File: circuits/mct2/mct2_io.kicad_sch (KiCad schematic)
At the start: 125 parts

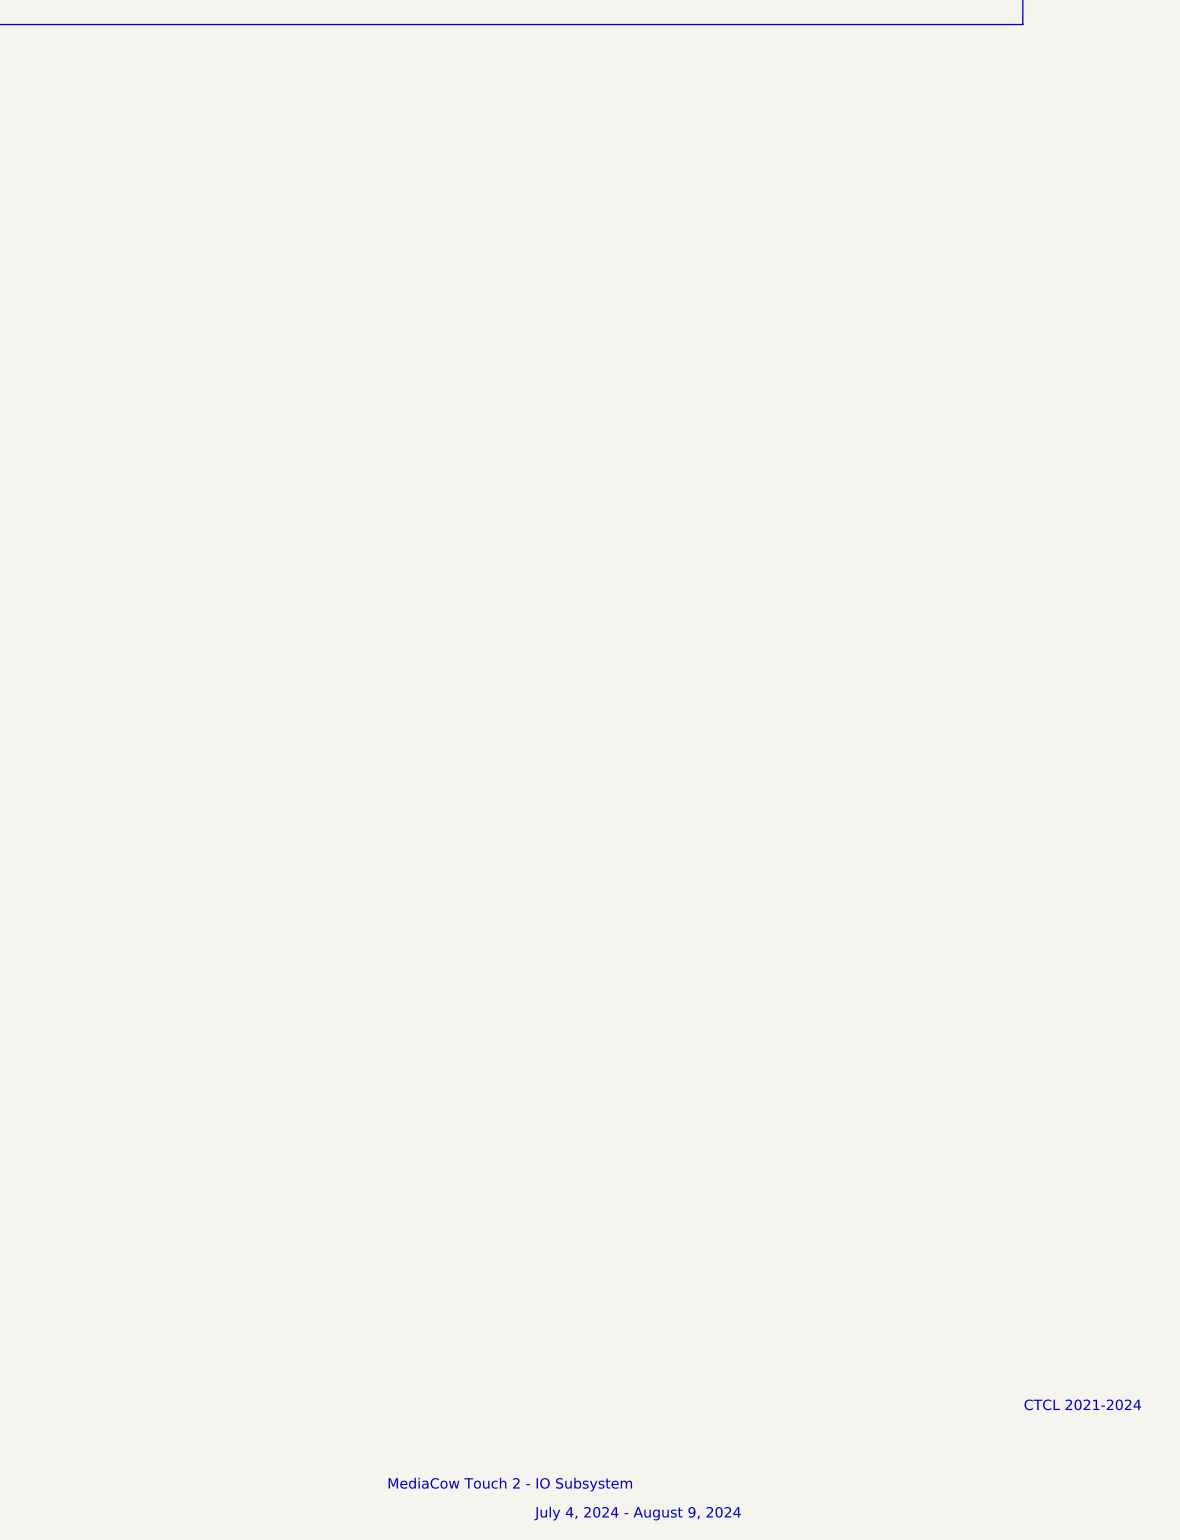
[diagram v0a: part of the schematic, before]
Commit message: Aug 11, 2024 2
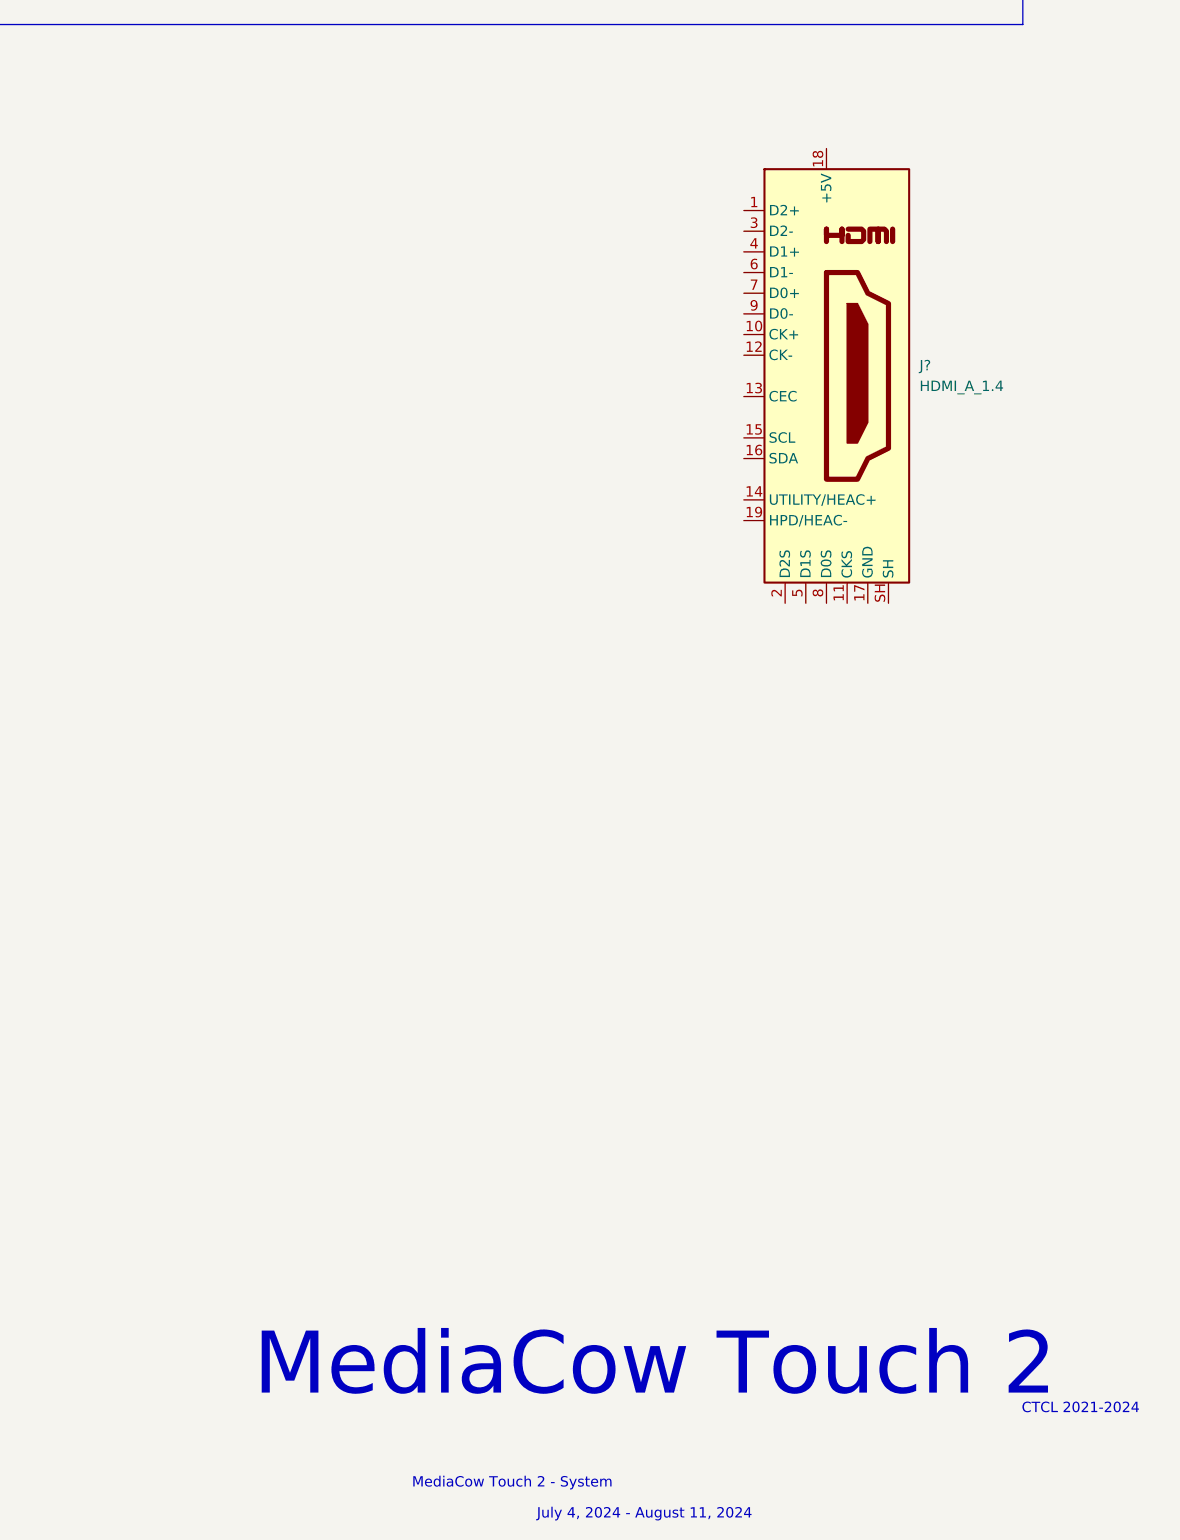
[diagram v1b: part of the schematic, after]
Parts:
- added J?: HDMI_A_1.4, symbol Connector:HDMI_A_1.4
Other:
- note added: "July 4, 2024 - August 11, 2024"
- note added: "MediaCow Touch 2"
- note added: "MediaCow Touch 2 - System"
- note removed: "July 4, 2024 - August 9, 2024"
- note removed: "MediaCow Touch 2 - IO Subsystem"
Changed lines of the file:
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@@
 		)
 	)
-	(text "July 4, 2024 - August 9, 2024"
+	(text "MediaCow Touch 2 - System"
 		(exclude_from_sim no)
-		(at 1113.536 824.484 0)
+		(at 1098.042 820.674 0)
 		(effects
 			(font
@@
 		)
 	)
-	(text "MediaCow Touch 2 - IO Subsystem\n"
+	(text "MediaCow Touch 2"
 		(exclude_from_sim no)
-		(at 1097.788 820.928 0)
+		(at 1115.568 806.196 0)
+		(effects
+			(font
+				(face "Heuristica")
+				(size 7.62 7.62)
+			)
+		)
+	)
+	(text "July 4, 2024 - August 11, 2024"
+		(exclude_from_sim no)
+		(at 1114.298 824.484 0)
 		(effects
 			(font
@@
 	(text "CTCL 2021-2024"
 		(exclude_from_sim no)
-		(at 1168.146 811.276 0)
+		(at 1167.892 811.53 0)
 		(effects
 			(font
@@
 					(unit 1)
 				)
+			)
+		)
+	)
+	(symbol
+		(lib_id "Connector:HDMI_A_1.4")
+		(at 1136.65 684.53 0)
+		(unit 1)
+		(exclude_from_sim no)
+		(in_bom yes)
+		(on_board yes)
+		(dnp no)
+		(fields_autoplaced yes)
+		(property "Reference" "J?"
+			(at 1148.08 683.2599 0)
+			(effects
+				(font
+					(size 1.27 1.27)
+				)
+				(justify left)
+			)
+		)
+		(property "Value" "HDMI_A_1.4"
+			(at 1148.08 685.7999 0)
+			(effects
+				(font
+					(size 1.27 1.27)
+				)
+				(justify left)
+			)
+		)
+		(property "Footprint" ""
+			(at 1137.285 684.53 0)
+			(effects
+				(font
+					(size 1.27 1.27)
+				)
+				(hide yes)
+			)
+		)
+		(property "Datasheet" "https://en.wikipedia.org/wiki/HDMI"
+			(at 1137.285 684.53 0)
+			(effects
+				(font
+					(size 1.27 1.27)
+				)
+				(hide yes)
+			)
+		)
+		(property "Description" "HDMI 1.4+ type A connector"
+			(at 1136.65 684.53 0)
+			(effects
+				(font
+					(size 1.27 1.27)
+				)
+				(hide yes)
+			)
+		)
+		(pin "14"
+		)
+		(pin "2"
+		)
+		(pin "9"
+		)
+		(pin "13"
+		)
+		(pin "SH"
+		)
+		(pin "1"
+		)
+		(pin "8"
+		)
+		(pin "18"
+		)
+		(pin "19"
+		)
+		(pin "12"
+		)
+		(pin "7"
+		)
+		(pin "10"
+		)
+		(pin "6"
+		)
+		(pin "11"
+		)
+		(pin "5"
+		)
+		(pin "15"
+		)
+		(pin "16"
+		)
+		(pin "17"
+		)
+		(pin "4"
+		)
+		(pin "3"
+		)
+		(instances
+			(project ""
+				(path "/0917e100-0497-47cd-9e32-3e43ad224d2b/c9720429-3bf3-4c3a-9e7d-2ba35698ba31"
+					(reference "J?")
+					(unit 1)
+				)

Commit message: Aug 13, 2024
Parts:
- removed C? (x4): 100nF, symbol Device:C_Small
- removed J?: USB_A_Stacked, symbol Connector:USB_A_Stacked
- removed R? (x2): 20K, symbol Device:R_Small
- removed R? (x2): 56K, symbol Device:R_Small
- removed U? (x2): TPS25221, symbol mediacow:TPS25221
- removed U? (x2): TPD4EUSB30, Package_TO_SOT_SMD:Texas_DRT-3, symbol mediacow:TPD2EUSB30
- added C? (x10): 220nF, symbol Device:C_Small
- added C? (x14): 100nF, symbol Device:C_Small
- added C? (x4): 10uF, symbol Device:C_Small
- added J?: Bus_M.2_Socket_E, symbol Connector:Bus_M.2_Socket_E
- added J?: Bus_M.2_Socket_M, symbol Connector:Bus_M.2_Socket_M
- added R? (x4): 0, symbol Device:R_Small
- added R? (x2): 10K, symbol Device:R_Small
- added U?: TPD4EUSB30, Package_TO_SOT_SMD:Texas_DRT-3, symbol mediacow:TPD2EUSB30
- added U?: TPD12S016RKTR, RKT24, symbol mediacow:TPD12S016RKTR
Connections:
- net GND: now also J?.11 (CKS), J?.17 (GND), J?.2 (D2S), J?.5 (D1S), J?.8 (D0S), J?.SH, C?.1, C?.1, C?.2, C?.2, C?.2, C?.2, C?.2, C?.2, C?.2, C?.2, J?.1 (GND), J?.1 (GND), J?.15 (GND), J?.18 (GND), J?.21 (GND), J?.27 (GND), J?.3 (GND), J?.33 (GND), J?.33 (GND), J?.39 (GND), J?.39 (GND), J?.45 (GND), J?.45 (GND), J?.51 (GND), J?.51 (GND), J?.57 (GND), J?.57 (GND), J?.63 (GND), J?.69 (GND), J?.7 (GND), J?.71 (GND), J?.73 (GND), J?.75 (GND), J?.75 (GND), J?.9 (GND), R?.1, R?.1, U?.13 (GND), U?.18 (GND), U?.3 (GND), U?.5 (GND)
- net LAN_0V9: now also U?.11 (VDD0p9), U?.32 (VDD0p9), U?.42 (VDD0p9), U?.59 (VDD0p9)
- net LAN_1V5: now also U?.47 (VDD1p5), U?.56 (VDD1p5)
- net at J?.1 (D2+): now also C?.1
- net at J?.10 (CK+): now also C?.1
- net at J?.12 (CK-): now also C?.1
- net DDIB_SCL_CN: now reaches J?.15 (SCL)
- net DDIB_SCL_CN: now also U?.7 (SCL_B)
- net DDIB_SDA_CN: now reaches J?.16 (SDA)
- net DDIB_SDA_CN: now also U?.8 (SDA_B)
- net DDIB_5V_CN: now reaches J?.18 (+5V)
- net DDIB_5V_CN: now also C?.2, U?.12 (5V_OUT)
- net DDIB_HPD_CN: now reaches J?.19 (HPD/HEAC-)
- net DDIB_HPD_CN: now also U?.9 (HPD_B)
- net at J?.3 (D2-): now also C?.1
- net at J?.4 (D1+): now also C?.1
- net at J?.6 (D1-): now also C?.1
- net at J?.7 (D0+): now also C?.1
- net at J?.9 (D0-): now also C?.1
- new net: J?.53 (~{CLKREQ0}), R?.2
- new net: C?.2, J?.37 (PETp1)
- new net: C?.2, J?.35 (PETn1)
- new net: C?.2, J?.13 (PETp3)
- new net: C?.2, J?.37 (PETn0)
- new net: J?.54 (~{W_DISABLE2}), R?.1
- new net: C?.2, J?.49 (PETp0/SATA-A+)
- new net: C?.2, J?.11 (PETn3)
- new net: J?.56 (~{W_DISABLE1}), R?.1
- new net: J?.68 (SUSCLK), R?.1
- new net: J?.50 (SUSCLK), R?.1
- new net: C?.2, J?.25 (PETp2)
- new net: J?.52 (~{CLKREQ}), R?.2
- new net: C?.2, J?.47 (PETn0/SATA-A-)
- new net: C?.2, J?.35 (PETp0)
- new net: C?.2, J?.23 (PETn2)
- new net DDIB_5V: C?.2, U?.10 (VCC5V)
- new net DDIB_HPD: U?.3 (HPD_A)
- new net DDIB_SCL: U?.1 (SCL_A)
- new net DDIB_SDA: U?.2 (SDA_A)
- new net DDIB_TX0_N: C?.2, U?.21 (D2-)
- new net DDIB_TX0_P: C?.2, U?.22 (D2+)
- new net DDIB_TX1_N: C?.2, U?.19 (D1-)
- new net DDIB_TX1_P: C?.2, U?.20 (D1+)
- new net DDIB_TX2_N: C?.2, U?.16 (D0-)
- new net DDIB_TX2_P: C?.2, U?.17 (D0+)
- new net DDIB_TX3_N: C?.2, U?.14 (CLK-)
- new net DDIB_TX3_P: C?.2, U?.15 (CLK+)
- new net PCIE_M2E_REF_N: J?.49 (REFCLKn0)
- new net PCIE_M2E_REF_P: J?.47 (REFCLKp0)
- new net PCIE_M2E_RX0_N: J?.43 (PERn0)
- new net PCIE_M2E_RX0_P: J?.41 (PERp0)
- new net PCIE_M2E_TX0_N: C?.1
- new net PCIE_M2E_TX0_P: C?.1
- new net PCIE_NVME_REF_N: J?.53 (REFCLKn)
- new net PCIE_NVME_REF_P: J?.55 (REFCLKp)
- new net PCIE_NVME_RX0_N: J?.41 (PERn0/SATA-B+)
- new net PCIE_NVME_RX0_P: J?.43 (PERp0/SATA-B-)
- new net PCIE_NVME_RX1_N: J?.29 (PERn1)
- new net PCIE_NVME_RX1_P: J?.31 (PERp1)
- new net PCIE_NVME_RX2_N: J?.17 (PERn2)
- new net PCIE_NVME_RX2_P: J?.19 (PERp2)
- new net PCIE_NVME_RX3_N: J?.5 (PERn3)
- new net PCIE_NVME_RX3_P: J?.7 (PERp3)
- new net PCIE_NVME_TX0_N: C?.1
- new net PCIE_NVME_TX0_P: C?.1
- new net PCIE_NVME_TX1_N: C?.1
- new net PCIE_NVME_TX1_P: C?.1
- new net PCIE_NVME_TX2_N: C?.1
- new net PCIE_NVME_TX2_P: C?.1
- new net PCIE_NVME_TX3_N: C?.1
- new net PCIE_NVME_TX3_P: C?.1
- new net PCIE_PLTRST: J?.50 (~{PERST}), J?.52 (~{PERST0})
- new net PCIE_WAKE: J?.54 (~{PEWAKE}), J?.55 (~{PEWAKE0})
- new net SMEC_3V3_IO: U?.23 (VCCA)
- new net SUSCLK: R?.2, R?.2
- new net SYS_3V3: C?.1, C?.1, C?.1, C?.1, C?.1, C?.1, C?.1, C?.1, J?.12 (3.3V), J?.14 (3.3V), J?.16 (3.3V), J?.18 (3.3V), J?.2 (3.3V), J?.2 (3.3V), J?.4 (3.3V), J?.4 (3.3V), J?.70 (3.3V), J?.72 (3.3V), J?.72 (3.3V), J?.74 (3.3V), J?.74 (3.3V), R?.2, R?.2
- new net USB_M2E_N: J?.5 (USB_D-), U?.2 (D1-)
- new net USB_M2E_P: J?.3 (USB_D+), U?.1 (D1+)
- no-connect marks 4 -> 42
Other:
- note added: "July 4, 2024 - August 13, 2024"
- note removed: "July 4, 2024 - August 11, 2024"
- moved on the sheet: C?, J?

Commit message: Aug 14, 2024 old stuff
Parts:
- removed JP?: ~, symbol Jumper:SolderJumper_3_Open
- added C?: 22pF, symbol Device:C_Small
- added C?: 2.2uF, symbol Device:C_Small
- added C?: 4.7uF, symbol Device:C_Small
- added C?: 22uF, symbol Device:C_Small
- added C?: 100nF, symbol Device:C_Small
- added D?: SS15, Diode_SMD:D_SMA, symbol Device:D_Schottky_Small_Filled
- added L?: 15uH, symbol Device:L_Small
- added NT?: NetTie_2, symbol Device:NetTie_2
- added R?: 100K, symbol Device:R_Small
- added R?: 22, symbol Device:R_Small
- added R?: 10K, symbol Device:R_Small
- added R?: 1M, symbol Device:R_Small
- added R?: 13.7K, symbol Device:R_Small
- added U?: SY21019, Package_TO_SOT_SMD:SOT-23-6, symbol mediacow:SY21019
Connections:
- net DDIB_TX0_N: no longer U?.21 (D2-)
- net DDIB_TX0_P: no longer U?.22 (D2+)
- net DDIB_TX1_N: no longer U?.19 (D1-)
- net DDIB_TX1_P: no longer U?.20 (D1+)
- net DDIB_TX2_N: no longer U?.16 (D0-)
- net DDIB_TX2_P: no longer U?.17 (D0+)
- net DDIB_TX3_N: no longer U?.14 (CLK-)
- net DDIB_TX3_P: no longer U?.15 (CLK+)
- net GND: now also C?.1, C?.2, C?.2, C?.2, D?.2 (A), NT?.2, R?.2, R?.2, U?.2 (GND); no longer C?.2, C?.2, C?.2
- net HDA_BCLK: now also R?.2
- net OLED_VDD: now also C?.1, C?.1, J?.5 (Pin_5), J?.7 (Pin_7)
- net VSYS: now also C?.1, C?.2, R?.1, U?.5 (IN)
- net DDIB_TX0_P_CN: now reaches C?.1, J?.1 (D2+)
- net DDIB_TX0_P_CN: now also U?.22 (D2+)
- net DDIB_TX3_P_CN: now reaches C?.1, J?.10 (CK+)
- net DDIB_TX3_P_CN: now also U?.15 (CLK+)
- net DDIB_TX3_N_CN: now reaches C?.1, J?.12 (CK-)
- net DDIB_TX3_N_CN: now also U?.14 (CLK-)
- net DDIB_TX0_N_CN: now reaches C?.1, J?.3 (D2-)
- net DDIB_TX0_N_CN: now also U?.21 (D2-)
- net DDIB_TX1_P_CN: now reaches C?.1, J?.4 (D1+)
- net DDIB_TX1_P_CN: now also U?.20 (D1+)
- net DDIB_TX1_N_CN: now reaches C?.1, J?.6 (D1-)
- net DDIB_TX1_N_CN: now also U?.19 (D1-)
- net DDIB_TX2_P_CN: now reaches C?.1, J?.7 (D0+)
- net DDIB_TX2_P_CN: now also U?.17 (D0+)
- net DDIB_TX2_N_CN: now reaches C?.1, J?.9 (D0-)
- net DDIB_TX2_N_CN: now also U?.16 (D0-)
- net CT_HPD: now reaches U?.11 (CT_HPD)
- net LS_OE: now reaches U?.4 (LS_OE)
- net HDA_DMIC_CLK: now reaches U?.2 (DMIC_CLK/GPIO_1)
- net HDA_DMIC_DAT: now reaches U?.3 (DMIC_0/GPIO_2)
- net DDIB_5V: no longer names the net of C?.2, U?.10 (VCC5V)
- net DDIB_5V: now also C?.1, L?.2, R?.1
- new net: C?.1, D?.1 (K), L?.1, U?.6 (LX)
- new net: C?.1, R?.1
- new net: R?.1, R?.2, U?.3 (FB)
- new net: R?.1, R?.2, U?.4 (EN)
- new net: C?.2, U?.1 (BS)
- new net CPVSS: C?.2, C?.2, C?.2, NT?.1
- no-connect marks 42 -> 44
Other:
- note added: "July 4, 2024 - August 14, 2024"
- note added: "OLED_VDD: 80XX GND: 68XX"
- note removed: "July 4, 2024 - August 13, 2024"
- moved on the sheet: C?, J?, J?A, JP?, R?, U?, Y?

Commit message: Aug 17, 2024
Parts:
- removed C? (x2): 10nF, symbol Device:C_Small
- removed C? (x4): 22uF, symbol Device:C_Small
- removed C? (x2): 100nF, symbol Device:C_Small
- removed C? (x4): 10uF, symbol Device:C_Small
- removed C?: 22pF, symbol Device:C_Small
- removed C?: 4.7uF, symbol Device:C_Small
- removed C?: 1uF, symbol Device:C_Small
- removed D?: B250A, symbol Device:D_Schottky_Small_Filled
- removed D?: MMSZ5231BS-7-F, Diode_SMD:D_SOD-323, symbol Device:D_Zener_Small_Filled
- removed L?: 15uH, symbol Device:L_Small
- removed L?: 2.2uH, symbol Device:L_Small
- removed R?: 100K, symbol Device:R_Small
- removed R? (x2): 0, symbol Device:R_Small
- removed R? (x3): 20K, symbol Device:R_Small
- removed R?: 220K, symbol Device:R_Small
- removed R?: 16K, symbol Device:R_Small
- removed R?: 150K, symbol Device:R_Small
- removed U?: RT6200, Package_TO_SOT_SMD:SOT-23-6, symbol mediacow:RT6200
- removed U?: TPS51386RJNR, VQFN-HR12_RJN_TEX, symbol mediacow:TPS51386RJNR
- added C? (x10): 100nF, symbol Device:C_Small
- added C?: 330nF, symbol Device:C_Small
- added C? (x2): 4.7uF, symbol Device:C_Small
- added C?: 1uF, symbol Device:C_Small
- added C? (x3): 2.2uF, symbol Device:C_Small
- added C? (x2): 22uF, symbol Device:C_Small
- added C? (x2): 10uF, symbol Device:C_Small
- added C?: 22pF, symbol Device:C_Small
- added D?: D_Schottky_Small_Filled, symbol Device:D_Schottky_Small_Filled
- added D? (x2): SS15, Diode_SMD:D_SMA, symbol Device:D_Schottky_Small_Filled
- added L?: 2.2uF, symbol Device:L_Small
- added L? (x2): 15uH, symbol Device:L_Small
- added R?: 430k, symbol Device:R_Small
- added R? (x2): 150, symbol Device:R_Small
- added R? (x2): 1M, symbol Device:R_Small
- added R? (x5): 10K, symbol Device:R_Small
- added R?: 5.23K, symbol Device:R_Small
- added R?: 4.99K, symbol Device:R_Small
- added R?: 22.1K, symbol Device:R_Small
- added R? (x4): 100K, symbol Device:R_Small
- added U?: L78L33_SO8, Package_SO:SOIC-8_3.9x4.9mm_P1.27mm, symbol Regulator_Linear:L78L33_SO8
- added U? (x2): SY21019, Package_TO_SOT_SMD:SOT-23-6, symbol mediacow:SY21019
- added U?: AP3401DN, mediacow:Diodes_U-DFN2020-6_Type_J, symbol mediacow:AP3401DN
- C?: value 1nF -> 1nF 2KV
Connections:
- net GND: now also C?.1, C?.1, C?.1, C?.1, C?.2, C?.2, C?.2, C?.2, C?.2, C?.2, C?.2, C?.2, C?.2, C?.2, C?.2, C?.2, C?.2, C?.2, C?.2, D?.2 (A), D?.2 (A), R?.1, R?.1, R?.1, R?.2, R?.2, R?.2, R?.2, R?.2, R?.2, U?.2 (GND), U?.2 (GND), U?.2 (GND), U?.3 (GND), U?.5 (GND), U?.6 (GND), U?.7 (GND)
- net OLED_VDD: now also C?.1, C?.2, L?.2, R?.1
- net OLED_VOLED: now also C?.1, C?.2, L?.2, R?.1
- net OLED_VOLED_EN: now also R?.1, R?.2, U?.4 (EN)
- net VSB: now also C?.1, C?.1, C?.2, C?.2, R?.1, R?.1, U?.5 (IN), U?.5 (IN)
- net at T?.1 (CT): now also C?.1
- net at T?.10 (CT): now also C?.1
- net LAN_MDI_3_P: now reaches T?.11 (TD4+)
- net LAN_MDI_3_P: now also U?.50 (MDI_PLUS[3]/SER_P)
- net LAN_MDI_3_N: now reaches T?.12 (TD4-)
- net LAN_MDI_3_N: now also U?.49 (MDI_MINUS[3]/SER_N)
- net LAN_MDI_0_P: now reaches T?.2 (TD1+)
- net LAN_MDI_0_P: now also U?.58 (MDI_PLUS[0]/NC)
- net LAN_MDI_0_N: now reaches T?.3 (TD1-)
- net LAN_MDI_0_N: now also U?.57 (MDI_MINUS[0]/SFP_I2C_DATA)
- net at T?.4 (CT): now also C?.1
- net LAN_MDI_1_P: now reaches T?.5 (TD2+)
- net LAN_MDI_1_P: now also U?.55 (MDI_PLUS[1]/SFP_I2C_CLK)
- net LAN_MDI_1_N: now reaches T?.6 (TD2-)
- net LAN_MDI_1_N: now also U?.54 (MDI_MINUS[1]/SRDS_SIG_DET)
- net at T?.7 (CT): now also C?.1
- net LAN_MDI_2_P: now reaches T?.8 (TD3+)
- net LAN_MDI_2_P: now also U?.53 (MDI_PLUS[2])
- net LAN_MDI_2_N: now reaches T?.9 (TD3-)
- net LAN_MDI_2_N: now also U?.52 (MDI_MINUS[2]/SET_N)
- net LAN_3V3: now reaches C?.1
- net LAN_3V3: now also C?.1, C?.1, C?.1, C?.1, J?.10, J?.12, U?.10 (VDD3p3), U?.27 (VDD3p3), U?.41 (VDD3p3), U?.51 (VDD3p3), U?.64 (VDD3p3), C?.1, C?.1, D?.2 (A), L?.2, R?.1
- net at U?.8 (VCC): now also C?.1, C?.1, D?.1 (K)
- net LAN_LINK: now reaches J?.11
- net LAN_LINK: now also R?.2
- net LAN_ACT: now reaches J?.9
- net LAN_ACT: now also R?.2
- net at U?.2 (NC_SI_CLK_IN): now also C?.1, R?.2
- net at U?.3 (NC_SI_CRS_DV): now also R?.2
- net at U?.30 (LED1): now also R?.1
- net at U?.33 (LED2): now also R?.1
- net at U?.48 (RSET): now also R?.1
- net at U?.7 (NC_SI_TX_EN): now also R?.2
- net M2M_DEVSLP: now reaches J?.38 (DEVSLP)
- net PCIE_NVME_REF_N renamed PCIE_M2M_REF_N
- net PCIE_NVME_REF_P renamed PCIE_M2M_REF_P
- net PCIE_NVME_RX0_N renamed PCIE_M2M_RX0_N
- net PCIE_NVME_RX0_P renamed PCIE_M2M_RX0_P
- net PCIE_NVME_RX1_N renamed PCIE_M2M_RX1_N
- net PCIE_NVME_RX1_P renamed PCIE_M2M_RX1_P
- net PCIE_NVME_RX2_N renamed PCIE_M2M_RX2_N
- net PCIE_NVME_RX2_P renamed PCIE_M2M_RX2_P
- net PCIE_NVME_RX3_N renamed PCIE_M2M_RX3_N
- net PCIE_NVME_RX3_P renamed PCIE_M2M_RX3_P
- net PCIE_NVME_TX0_N renamed PCIE_M2M_TX0_N
- net PCIE_NVME_TX0_P renamed PCIE_M2M_TX0_P
- net PCIE_NVME_TX1_N renamed PCIE_M2M_TX1_N
- net PCIE_NVME_TX1_P renamed PCIE_M2M_TX1_P
- net PCIE_NVME_TX2_N renamed PCIE_M2M_TX2_N
- net PCIE_NVME_TX2_P renamed PCIE_M2M_TX2_P
- net PCIE_NVME_TX3_N renamed PCIE_M2M_TX3_N
- net PCIE_NVME_TX3_P renamed PCIE_M2M_TX3_P
- new net: C?.2, R?.1, R?.2, U?.6 (FB)
- new net: C?.1, U?.1 (OUT)
- new net: C?.1, D?.1 (K), L?.1, U?.6 (LX) (x2)
- new net: C?.2, U?.1 (BS) (x2)
- new net: L?.1, U?.4 (LX)
- new net: R?.1, R?.2, U?.3 (FB) (x2)
- new net: R?.2, U?.2 (PG)
- new net OLED_VDD_EN: R?.1, R?.2, U?.4 (EN)
- new net VSYS_LV: C?.1, C?.1, R?.1, U?.1 (EN), U?.3 (VIN), U?.8 (IN)
- no-connect marks 44 -> 50
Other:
- note added: "July 4, 2024 - August 17, 2024"
- note removed: "12v"
- note removed: "July 4, 2024 - August 14, 2024"
- moved on the sheet: C?, J?, JP?, R?, T?, Y?
